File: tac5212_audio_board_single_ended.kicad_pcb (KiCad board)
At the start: 4 copper layers, 42 x 26.5 mm, 94 parts, among them J1002 TAC5212, U1 Single Buffer - 74LVC1G125GV,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, U2 3.3v LDO - TLV74133PDBVR

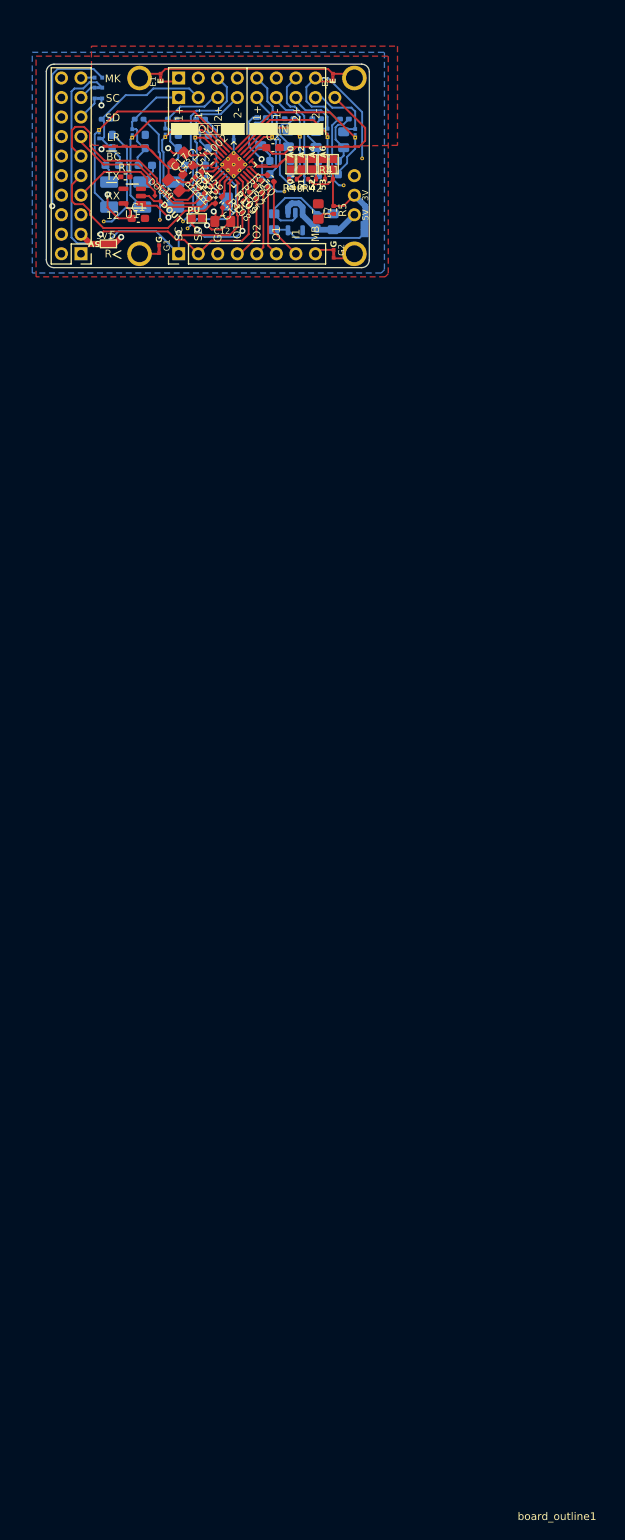
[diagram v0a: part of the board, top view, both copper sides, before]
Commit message: UPDATE
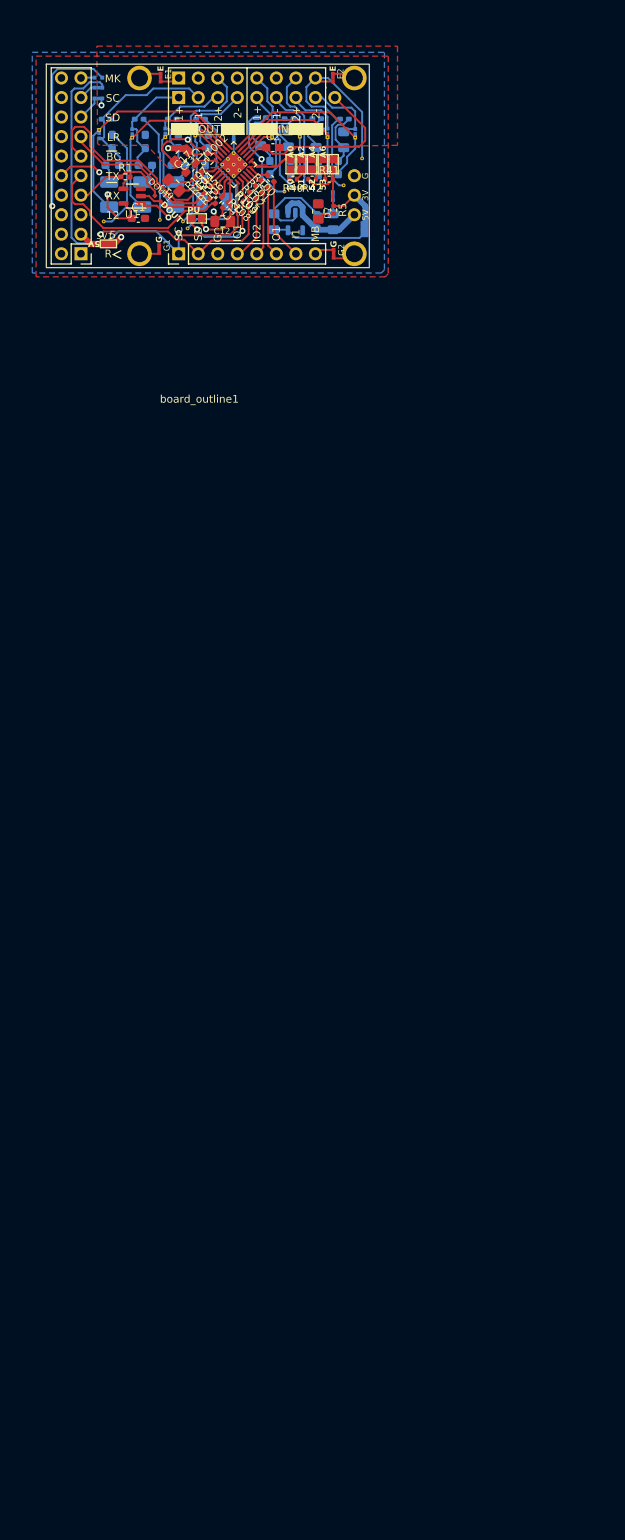
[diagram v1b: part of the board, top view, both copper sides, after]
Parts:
- added G108: jumper, project_fp:jumper_slice, B.Cu at (122.1, 115.1)
- moved C17 0.50 mm to (103.6, 111.4)
- moved C15 0.46 mm to (105.6, 109.2)
- moved C13 0.42 mm to (102.4, 109.9)
- moved OM2 0.30 mm to (104.2, 106.7)
- turned E1 to 90 degrees
- turned E2 to 90 degrees
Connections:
- E1 pad 1: Net-(E1-A) -> Earth
- E1 pad 2: Earth -> Net-(E1-B)
- E2 pad 1: Net-(E2-A) -> Earth
- E2 pad 2: Earth -> Net-(E2-B)
- T*C1 pad 2: GNDD -> Net-(G108-A)
- T*C2 pad 2: GNDD -> Net-(G108-A)
- T*C3 pad 2: GNDD -> Net-(G108-A)
- U2 pad 2: GNDD -> Net-(G108-A)
- board_outline1 pad 49: Net-(E1-A) -> Net-(E1-B)
- board_outline1 pad 50: Net-(E2-A) -> Net-(E2-B)
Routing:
- net (no net): track 28.9 -> 0.00 mm
- net GNDD: track 42.7 -> 21.9 mm
- net Net-(G108-A): track 0.00 -> 15.5 mm
- net Earth: track 157.7 -> 167.5 mm, vias 1 -> 2
- net Net-(E2-B): track 0.00 -> 3.02 mm
- net Net-(E1-B): track 0.00 -> 2.97 mm
- net Net-(U1-Y): track 0.00 -> 1.90 mm
- net 3.3V_LDO: track 90.1 -> 91.4 mm
- net Net-(J1002-VREF): track 3.46 -> 2.85 mm
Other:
- outline, holes or cut-outs redrawn
